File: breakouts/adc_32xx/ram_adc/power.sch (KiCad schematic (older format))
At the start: 13 parts, among them J501 Conn_01x01, J502 Conn_01x01, U501 ADM7170

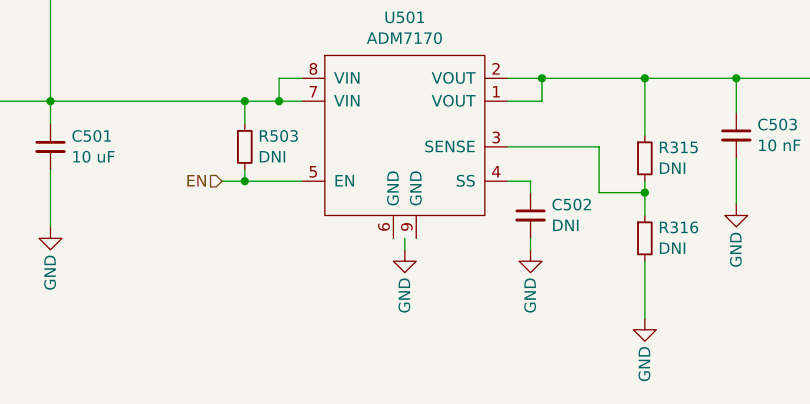
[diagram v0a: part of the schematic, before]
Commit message: finished layout of adc32xx ecp5 board
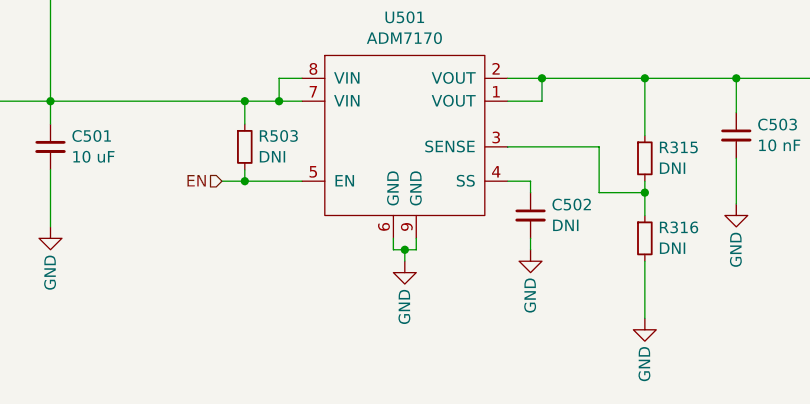
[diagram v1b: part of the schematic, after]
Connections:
- net GND: now also U501.6 (GND), U501.9 (GND)
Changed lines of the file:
@@
 L power:GND #PWR?
 U 1 1 5ED1D65E
-P 3800 4200
+P 3800 4250
 AR Path="/5ED1D65E" Ref="#PWR?"  Part="1"
 AR Path="/5E9D7371/5ED1D65E" Ref="#PWR?"  Part="1"
 AR Path="/5ED11961/5ED1D65E" Ref="#PWR0504"  Part="1"
-F 0 "#PWR0504" H 3800 3950 50  0001 C CNN
-F 1 "GND" V 3800 4000 50  0000 C CNN
-F 2 "" H 3800 4200 50  0001 C CNN
-F 3 "" H 3800 4200 50  0001 C CNN
-	1    3800 4200
-	1    0    0    -1
-$EndComp
-Wire Wire Line
-	3800 4150 3800 4200
+F 0 "#PWR0504" H 3800 4000 50  0001 C CNN
+F 1 "GND" V 3800 4050 50  0000 C CNN
+F 2 "" H 3800 4250 50  0001 C CNN
+F 3 "" H 3800 4250 50  0001 C CNN
+	1    3800 4250
+	1    0    0    -1
+$EndComp
+Wire Wire Line
+	3800 4200 3800 4250
 $Comp
 L power:GND #PWR?
@@
 Wire Wire Line
 	4850 3450 5250 3450
+Wire Wire Line
+	3750 4150 3750 4200
+Wire Wire Line
+	3750 4200 3800 4200
+Wire Wire Line
+	3800 4200 3850 4200
+Wire Wire Line
+	3850 4200 3850 4150
+Connection ~ 3800 4200
 $EndSCHEMATC
